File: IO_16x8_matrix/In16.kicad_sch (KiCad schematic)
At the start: 6 parts, among them J7 Conn_01x09, J8 Conn_01x10, J9 Conn_01x10

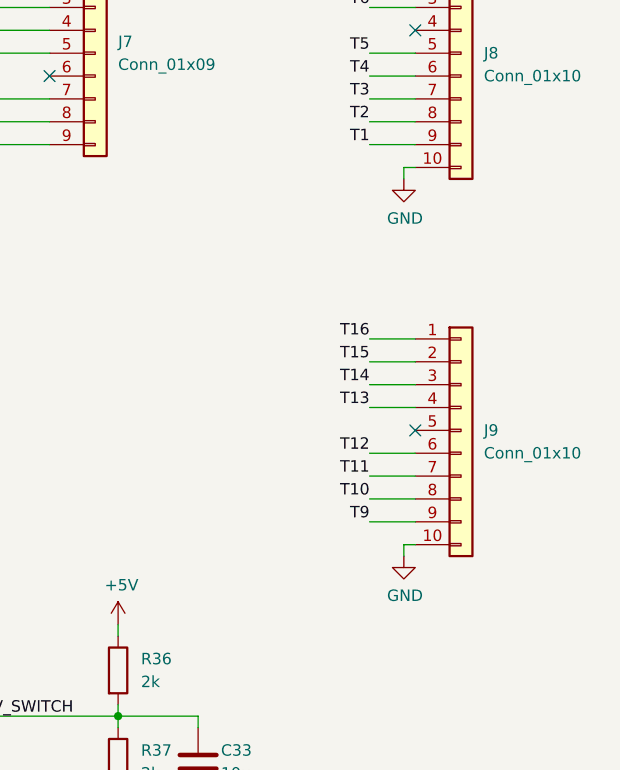
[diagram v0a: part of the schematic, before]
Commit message: routed
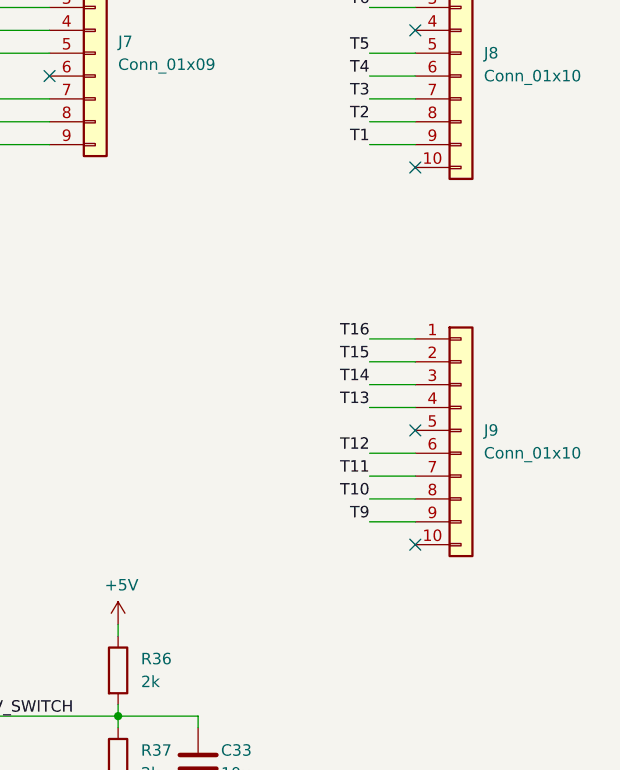
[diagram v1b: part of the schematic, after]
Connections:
- net GND: no longer J8.10 (Pin_10), J9.10 (Pin_10)
- no-connect marks 3 -> 5
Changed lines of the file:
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@@
   (junction (at 209.55 118.11) (diameter 0) (color 0 0 0 0)
   )
+  (no_connect (at 242.57 57.15))
   (no_connect (at 242.57 41.91))
   (no_connect (at 201.93 46.99))
   (no_connect (at 242.57 86.36))
+  (no_connect (at 242.57 99.06))
   (wire (pts (xy 194.31 54.61) (xy 201.93 54.61))
     (stroke (width 0) (type default) (color 0 0 0 0))
@@
     (stroke (width 0) (type default) (color 0 0 0 0))
   )
-  (wire (pts (xy 241.3 57.15) (xy 241.3 58.42))
-    (stroke (width 0) (type default) (color 0 0 0 0))
-  )
   (wire (pts (xy 237.49 96.52) (xy 242.57 96.52))
     (stroke (width 0) (type default) (color 0 0 0 0))
@@
     (stroke (width 0) (type default) (color 0 0 0 0))
   )
-  (wire (pts (xy 242.57 99.06) (xy 241.3 99.06))
-    (stroke (width 0) (type default) (color 0 0 0 0))
-  )
   (wire (pts (xy 106.68 36.83) (xy 113.03 36.83))
     (stroke (width 0) (type default) (color 0 0 0 0))
@@
     (stroke (width 0) (type default) (color 0 0 0 0))
   )
-  (wire (pts (xy 242.57 57.15) (xy 241.3 57.15))
-    (stroke (width 0) (type default) (color 0 0 0 0))
-  )
   (wire (pts (xy 31.75 44.45) (xy 38.1 44.45))
     (stroke (width 0) (type default) (color 0 0 0 0))
@@
   )
   (wire (pts (xy 106.68 121.92) (xy 113.03 121.92))
-    (stroke (width 0) (type default) (color 0 0 0 0))
-  )
-  (wire (pts (xy 241.3 99.06) (xy 241.3 100.33))
     (stroke (width 0) (type default) (color 0 0 0 0))
   )
@@
   (hierarchical_label "RTN_13" (shape output) (at 106.68 106.68 180)
     (effects (font (size 1.27 1.27)) (justify right))
-  )
-  (symbol (lib_id "power:GND") (at 241.3 100.33 0) (unit 1)
-    (in_bom yes) (on_board yes)
-    (property "Reference" "#PWR032" (id 0) (at 241.3 106.68 0)
-      (effects (font (size 1.27 1.27)) hide)
-    )
-    (property "Value" "GND" (id 1) (at 241.427 104.7242 0))
-    (property "Footprint" "" (id 2) (at 241.3 100.33 0)
-      (effects (font (size 1.27 1.27)) hide)
-    )
-    (property "Datasheet" "" (id 3) (at 241.3 100.33 0)
-      (effects (font (size 1.27 1.27)) hide)
-    )
-    (pin "1")
   )
   (symbol (lib_id "Device:R") (at 209.55 123.19 0) (unit 1)
@@
       (effects (font (size 1.27 1.27)) hide)
     )
-    (pin "1")
-  )
-  (symbol (lib_id "power:GND") (at 241.3 58.42 0) (unit 1)
-    (in_bom yes) (on_board yes)
-    (property "Reference" "#PWR031" (id 0) (at 241.3 64.77 0)
-      (effects (font (size 1.27 1.27)) hide)
-    )
-    (property "Value" "GND" (id 1) (at 241.427 62.8142 0))
-    (property "Footprint" "" (id 2) (at 241.3 58.42 0)
-      (effects (font (size 1.27 1.27)) hide)
-    )
-    (property "Datasheet" "" (id 3) (at 241.3 58.42 0)
-      (effects (font (size 1.27 1.27)) hide)
-    )

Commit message: opt routing
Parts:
- J7: now left out of the parts list
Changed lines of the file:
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@@
   )
   (symbol (lib_id "Connector_Generic:Conn_01x09") (at 207.01 44.45 0) (unit 1)
-    (in_bom yes) (on_board yes) (fields_autoplaced)
+    (in_bom no) (on_board yes) (fields_autoplaced)
     (property "Reference" "J7" (id 0) (at 209.55 43.1799 0)
       (effects (font (size 1.27 1.27)) (justify left))
